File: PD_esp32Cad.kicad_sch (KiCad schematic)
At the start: 27 parts, among them J1 USB_C_Receptacle_USB2.0_14P, SW1 reset, SW2 BOOT, U1 ESP32-S3-WROOM-1, U2 LM5148RGYR, U4 AP63203WU, U5 CYPD3177-24LQ

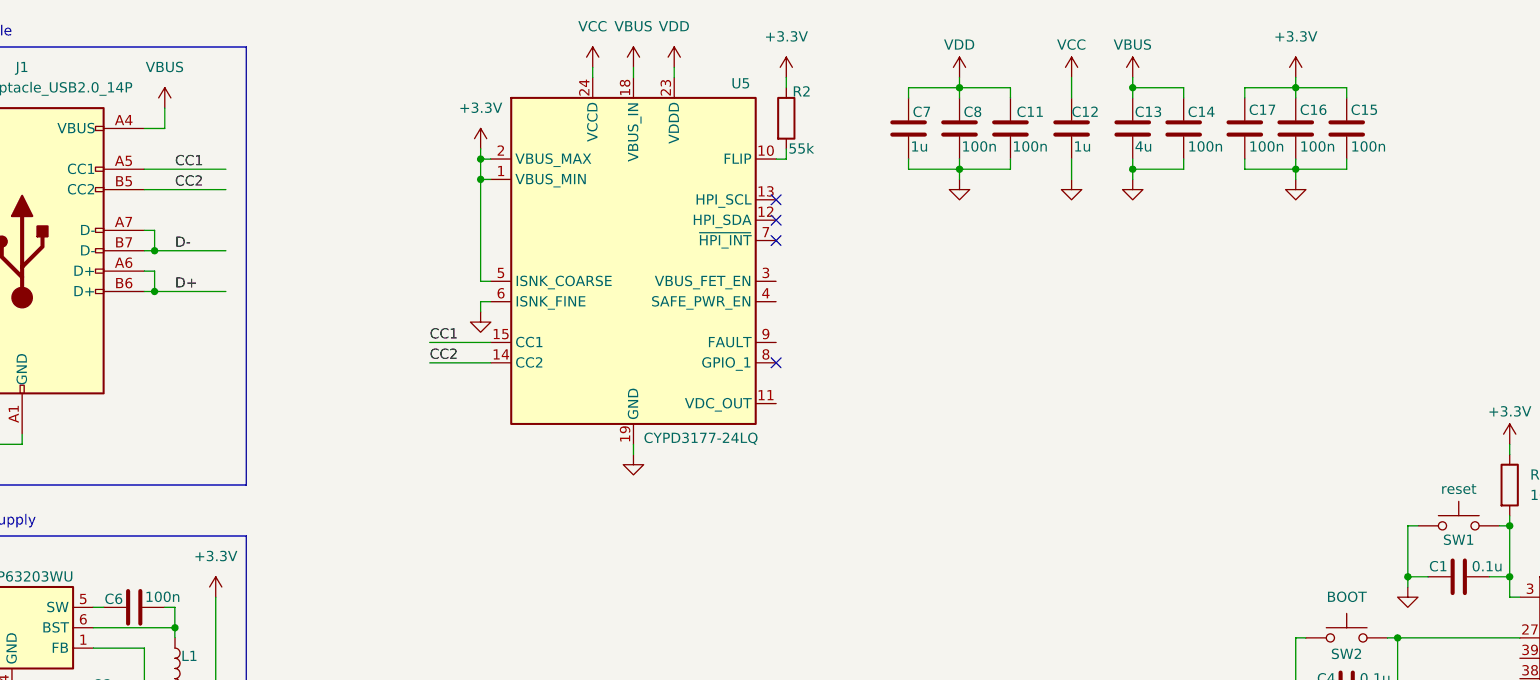
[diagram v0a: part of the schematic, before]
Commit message: PD_sink
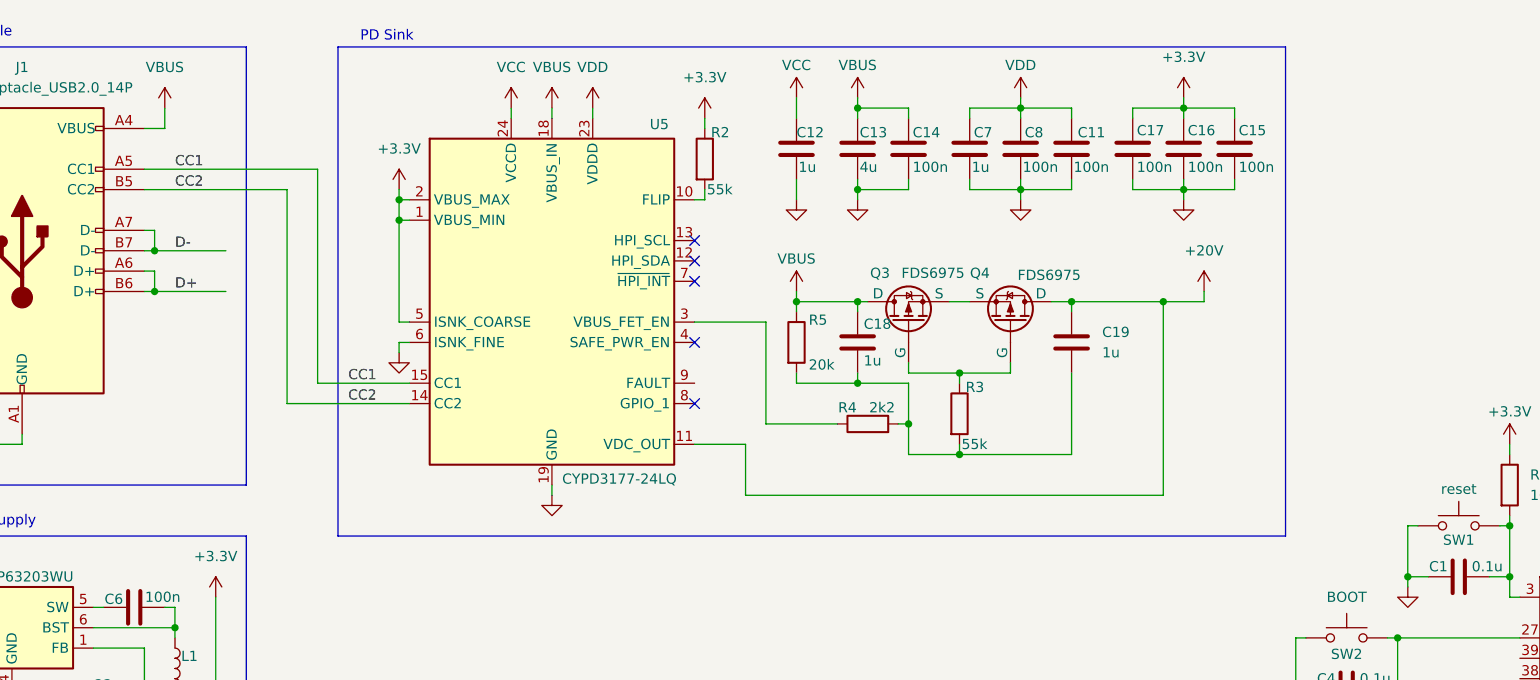
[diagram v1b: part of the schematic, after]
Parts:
- added C18, C19: 1u, symbol Device:C
- added Q3, Q4: FDS6975, symbol Simulation_SPICE:PMOS
- added R3: 55k, symbol Device:R
- added R4: 2k2, symbol Device:R
- added R5: 20k, symbol Device:R
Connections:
- net VBUS: now also C18.1, Q3.1 (D), R5.1
- net +20V: now reaches U5.11 (VDC_OUT)
- net +20V: now also C19.1, Q4.1 (D)
- net at U5.3 (VBUS_FET_EN): now also R4.1
- new net: Q3.2 (G), Q4.2 (G), R3.1
- new net: C18.2, C19.2, R3.2, R4.2, R5.2
- new net: Q3.3 (S), Q4.3 (S)
- no-connect marks 4 -> 5
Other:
- note added: "PD Sink"
- moved on the sheet: C11, C12, C13, C14, C15, C16, C17, C7, C8, R2, U5
